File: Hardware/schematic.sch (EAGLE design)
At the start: 103 parts, among them IC1 BD5229G-TR, IC4 XC6220A331MR-G, J1 FH34SRJ-24S-0.5SH_99_, J2 SAMACSYS_PARTS_USB4110-GF-A, J3 QWIIC_RIGHT_ANGLE, J4 112A-TAAR-R03_ATTEND, Q1 20V/4.2A/52mΩ/1.4W, Q2 20V/4.2A/52mΩ/1.4W, Q3 SI1308EDL-T1-GE3, U1 W25Q512JVEIQ, U2 ESP32-C6-WROOM-1-N8, U3 DS3231SN#, U4 MAX17048G+T10

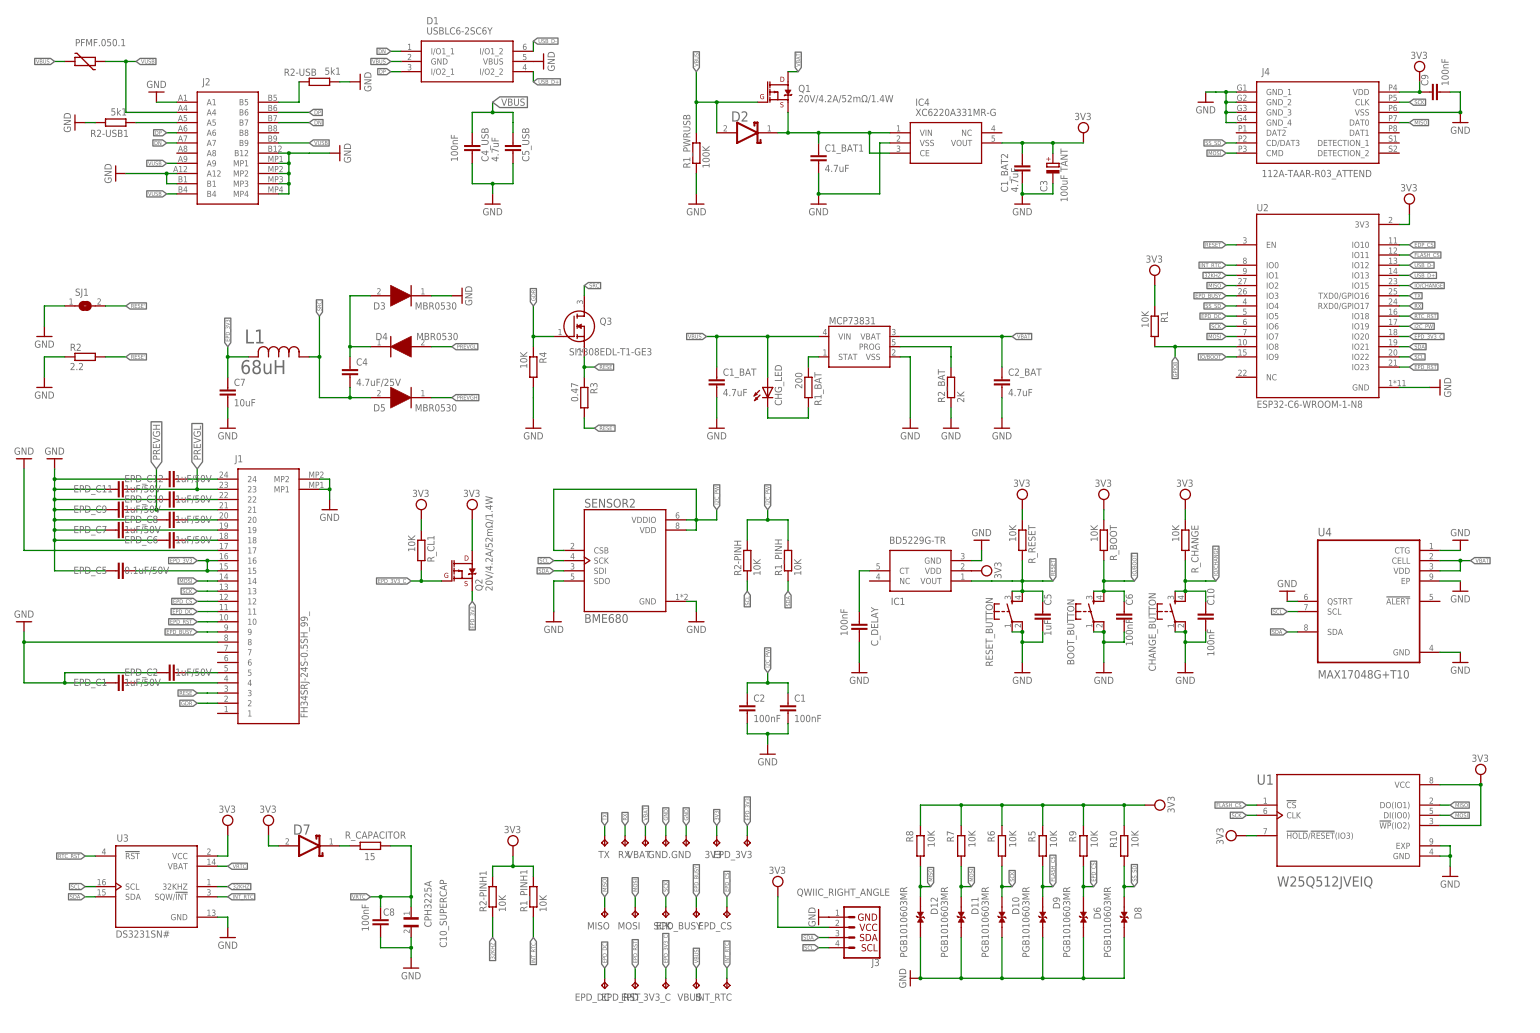
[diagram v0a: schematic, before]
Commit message: add files
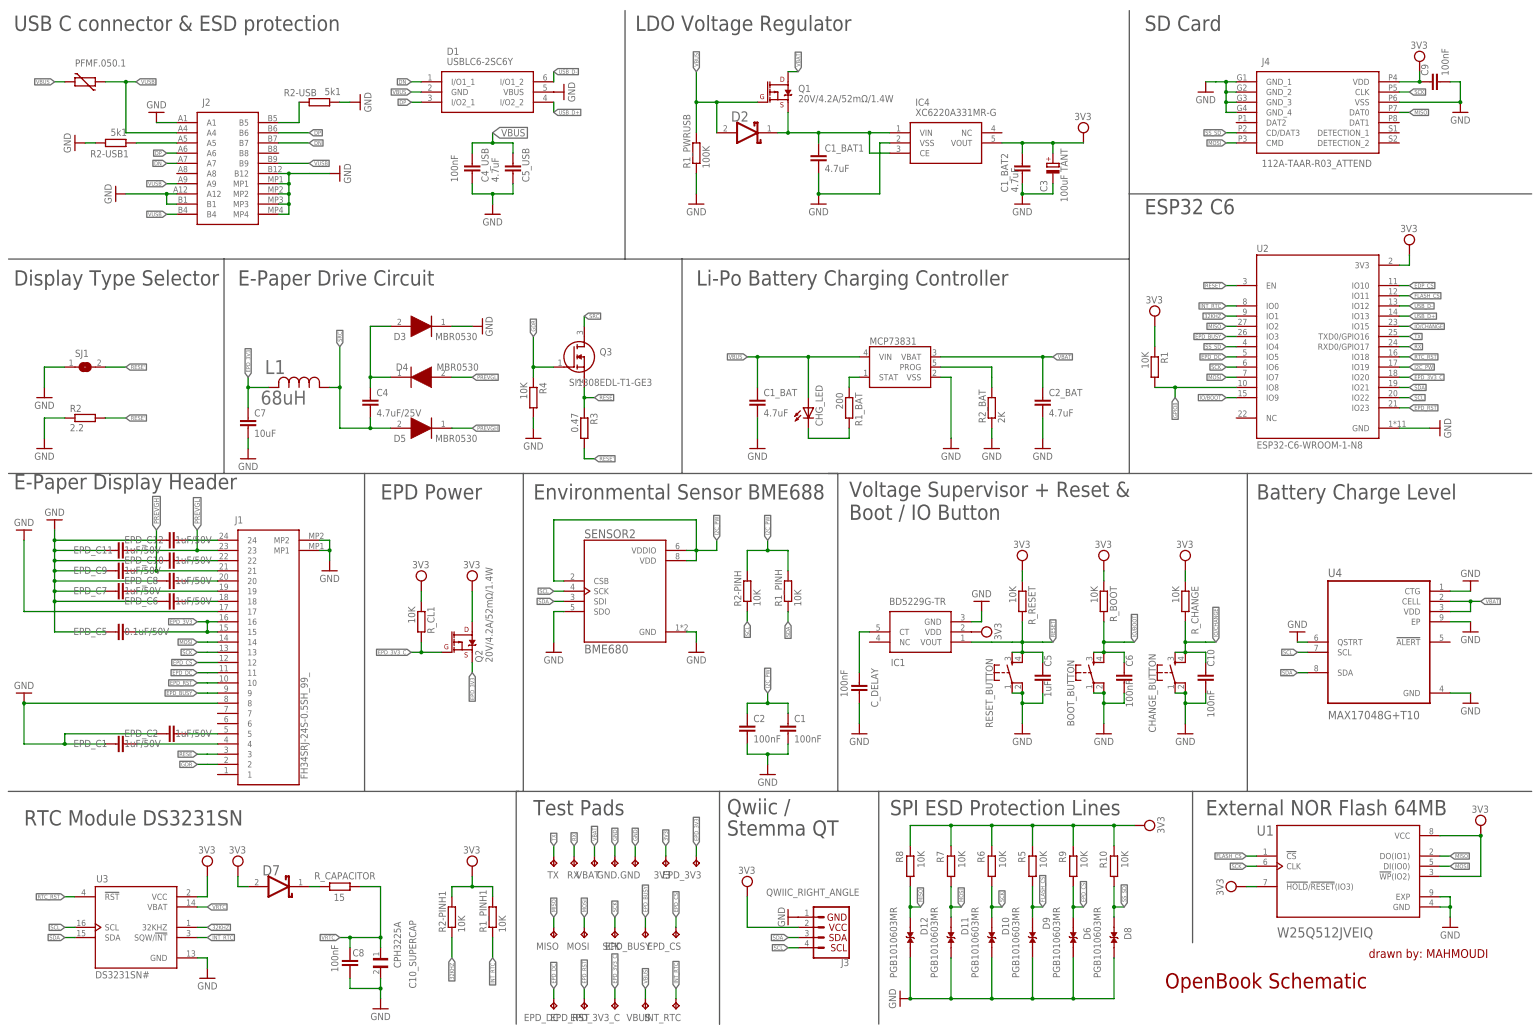
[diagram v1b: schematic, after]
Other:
- note added: "Battery Charge Level"
- note added: "Display Type Selector"
- note added: "E-Paper Display Header"
- note added: "E-Paper Drive Circuit"
- note added: "EPD Power"
- note added: "ESP32 C6"
- note added: "Environmental Sensor BME688"
- note added: "External NOR Flash 64MB"
- note added: "LDO Voltage Regulator"
- note added: "Li-Po Battery Charging Controller"
- note added: "OpenBook Schematic"
- note added: "Qwiic / Stemma QT"
- note added: "RTC Module DS3231SN"
- note added: "SD Card"
- note added: "SPI ESD Protection Lines"
- note added: "Test Pads"
- note added: "USB C connector & ESD protection"
- note added: "Voltage Supervisor + Reset & Boot / IO Button"
- note added: "drawn by: MAHMOUDI"
- moved on the sheet: 3V3, BOOT_BUTTON, C1, C10, C10_SUPERCAP, C1_BAT, C2, C2_BAT, C4, C4_USB, C5, C5_USB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
